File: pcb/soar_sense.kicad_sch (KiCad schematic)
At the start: 39 parts, among them J1 Conn_02x03_Top_Bottom, J2 Conn_02x02_Top_Bottom, J3 Conn_02x02_Top_Bottom, J4 Conn_02x02_Top_Bottom, J5 Conn_02x02_Top_Bottom, J6 Conn_02x01, J7 Conn_02x03_Top_Bottom, J8 Conn_02x04_Top_Bottom, U1 SPX3819M5-L-3-3, U2 STM32F103CBTx, U3 SHT35-DIS, U4 MAX3051, Y1 8MHz

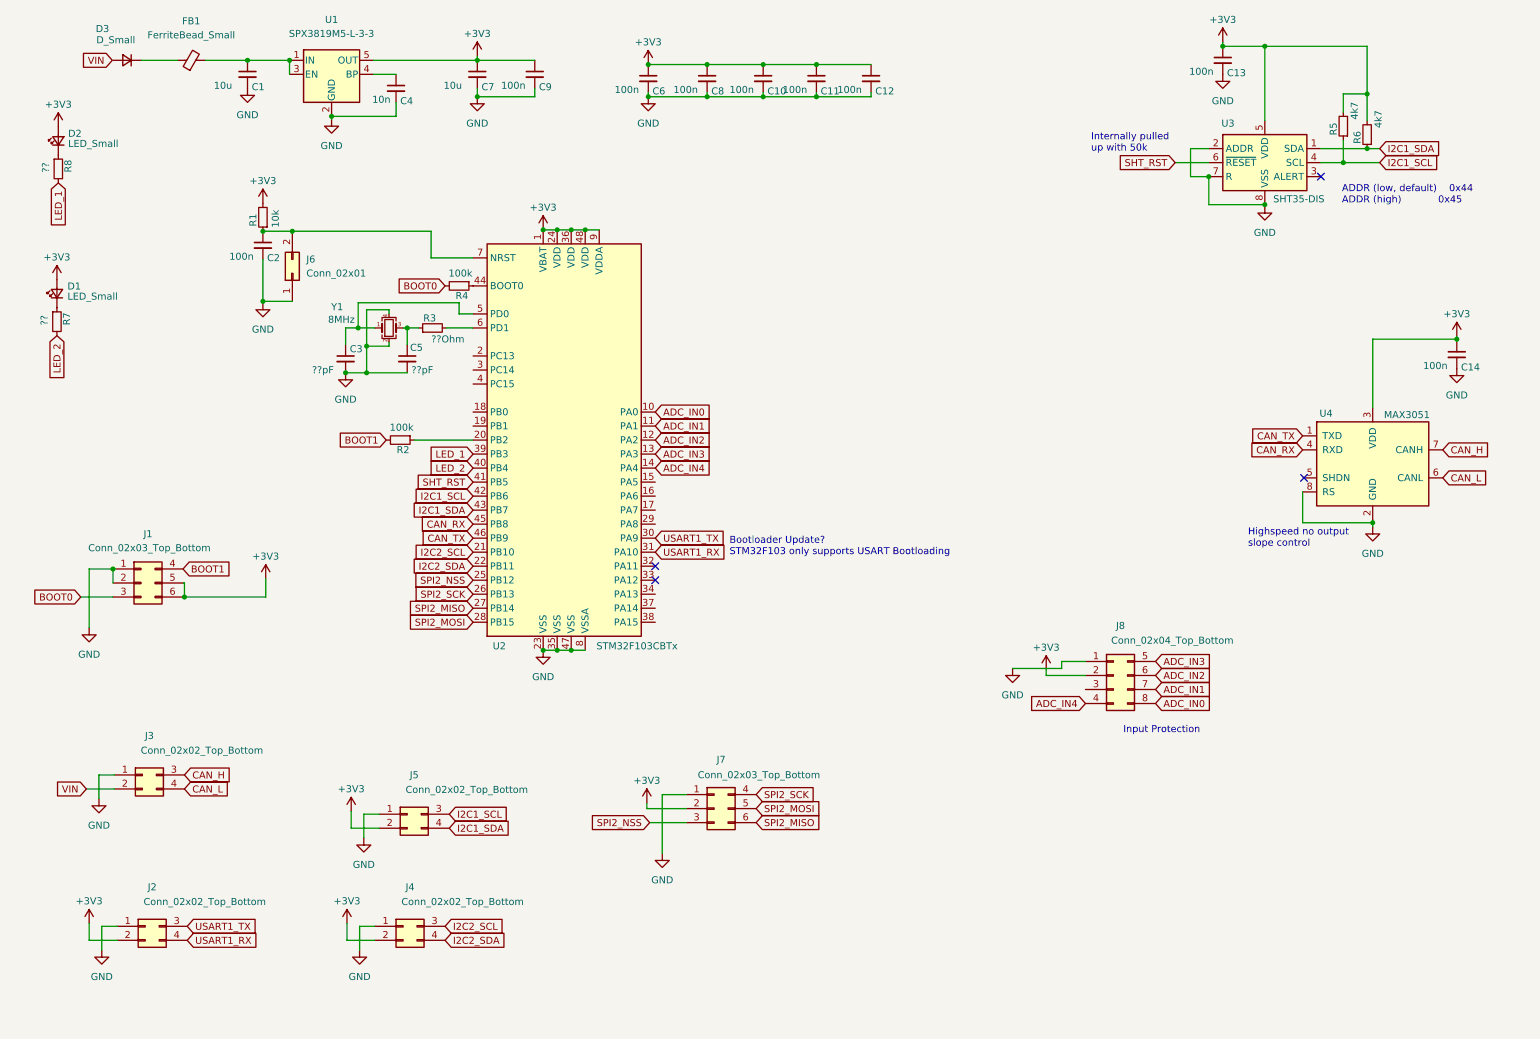
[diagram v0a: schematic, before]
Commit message: today done
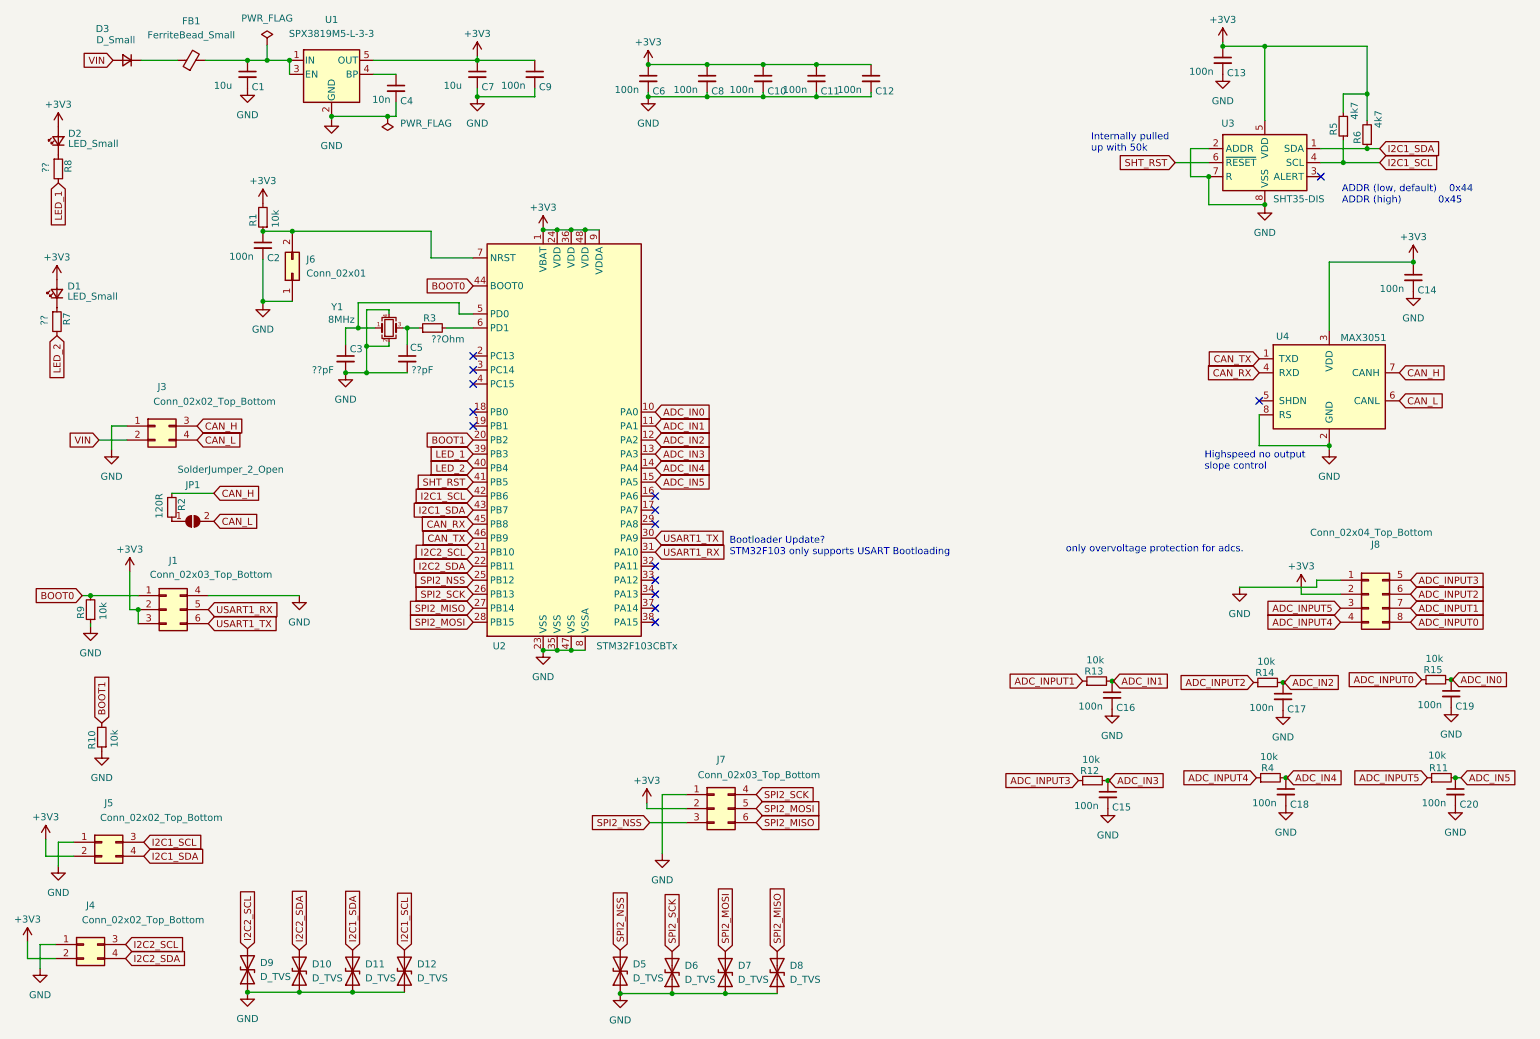
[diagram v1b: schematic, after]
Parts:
- removed J2: Conn_02x02_Top_Bottom, OWN_Parts:pcb_edge_2_2, symbol Connector_Generic:Conn_02x02_Top_Bottom
- added C15, C16, C17, C18, C19, C20: 100n, Capacitor_SMD:C_0603_1608Metric, symbol Device:C_Small
- added D10, D11, D12, D5, D6, D7, D8, D9: D_TVS, Diode_SMD:D_SOD-323, symbol Device:D_TVS
- added JP1: SolderJumper_2_Open, Jumper:SolderJumper-2_P1.3mm_Open_Pad1.0x1.5mm, symbol Jumper:SolderJumper_2_Open
- added R10, R11, R12, R13, R14, R15, R9: 10k, Resistor_SMD:R_0603_1608Metric, symbol Device:R_Small
- C10, C11, C12, C13, C14, C2, C6, C8, C9: LCSC Part Number (none) -> C14663
- C4: LCSC Part Number (none) -> C57112
- FB1: LCSC Part Number (none) -> C1017
- R1: LCSC Part Number (none) -> C25804
- R2: value 100k -> 120R; LCSC Part Number (none) -> C22787
- R4: value 100k -> 10k
- R5, R6: LCSC Part Number (none) -> C23162
- Y1: footprint (none) -> Crystal:Crystal_SMD_3225-4Pin_3.2x2.5mm
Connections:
- net +3V3: now also J1.2 (Pin_2), J1.3 (Pin_3); no longer J1.5 (Pin_5), J1.6 (Pin_6)
- net ADC_IN0: now also C19.1, R15.2; no longer J8.8 (Pin_8)
- net ADC_IN1: now also C16.1, R13.2; no longer J8.7 (Pin_7)
- net ADC_IN2: now also C17.1, R14.2; no longer J8.6 (Pin_6)
- net ADC_IN3: now also C15.1, R12.2; no longer J8.5 (Pin_5)
- net ADC_IN4: now also R4.2, C18.1; no longer J8.4 (Pin_4)
- net BOOT0: now also J1.1 (Pin_1), U2.44 (BOOT0), R9.2; no longer J1.3 (Pin_3), R4.2
- net BOOT1: now also U2.20 (PB2), R10.2; no longer J1.4 (Pin_4), R2.2
- net CAN_H: now also R2.1
- net CAN_L: now also JP1.2 (B)
- net GND: now also J1.4 (Pin_4), C15.2, C16.2, C17.2, C18.2, C19.2, C20.2, D10.1 (A1), D11.1 (A1), D12.1 (A1), D5.1 (A1), D6.1 (A1), D7.1 (A1), D8.1 (A1), D9.1 (A1), R10.1, R9.1; no longer J1.1 (Pin_1), J1.2 (Pin_2)
- net I2C1_SCL: now also D12.2 (A2)
- net I2C1_SDA: now also D11.2 (A2)
- net I2C2_SCL: now also D9.2 (A2)
- net I2C2_SDA: now also D10.2 (A2)
- net SPI2_MISO: now also D8.2 (A2)
- net SPI2_MOSI: now also D7.2 (A2)
- net SPI2_NSS: now also D5.2 (A2)
- net SPI2_SCK: now also D6.2 (A2)
- net USART1_RX: now also J1.5 (Pin_5)
- net USART1_TX: now also J1.6 (Pin_6)
- net VIN: now also D3.2 (A)
- net ADC_INPUT4: now reaches R4.1
- net ADC_INPUT4: now also J8.4 (Pin_4); no longer U2.44 (BOOT0)
- net ADC_INPUT5: now reaches J8.3 (Pin_3)
- net ADC_INPUT5: now also R11.1
- net ADC_IN5: now reaches U2.15 (PA5)
- net ADC_IN5: now also C20.1, R11.2
- new net: JP1.1 (A), R2.2
- new net ADC_INPUT0: J8.8 (Pin_8), R15.1
- new net ADC_INPUT1: J8.7 (Pin_7), R13.1
- new net ADC_INPUT2: J8.6 (Pin_6), R14.1
- new net ADC_INPUT3: J8.5 (Pin_5), R12.1
- no-connect marks 4 -> 15
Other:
- note added: "only overvoltage protection for adcs."
- note removed: "Input Protection"
- moved on the sheet: C14, J1, J3, J4, J5, J8, U4
